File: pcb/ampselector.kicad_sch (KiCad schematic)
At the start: 24 parts, among them SW1 SW_Push, SW10 RotaryEncoder_Switch, SW2 SW_Push, SW3 SW_Push, SW4 SW_Push, SW5 SW_Push, SW6 SW_Push, SW7 SW_Push, SW8 SW_Push, SW9 RotaryEncoder_Switch, U1 MOUDLE-SEEEDUINO-XIAO, U2 ER_OLEDM0.91_1x-I2C

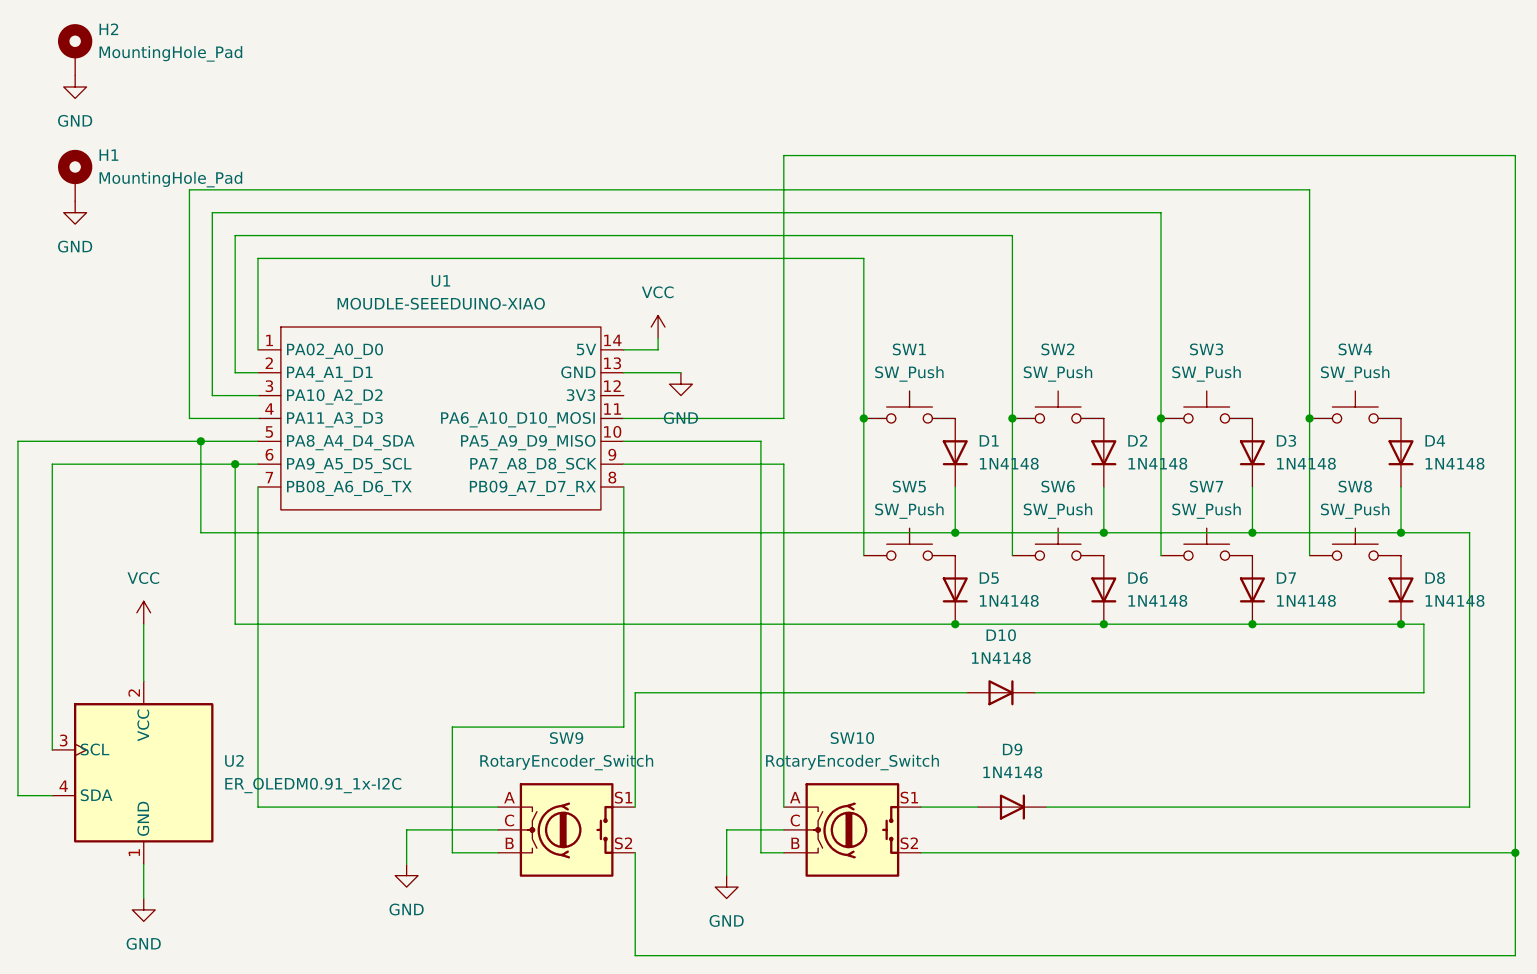
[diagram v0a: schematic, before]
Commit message: Designed Case
Signed-off-by: Ravinder Olivier Singh Dadiala <ravinder-Olivier@outlook.com>
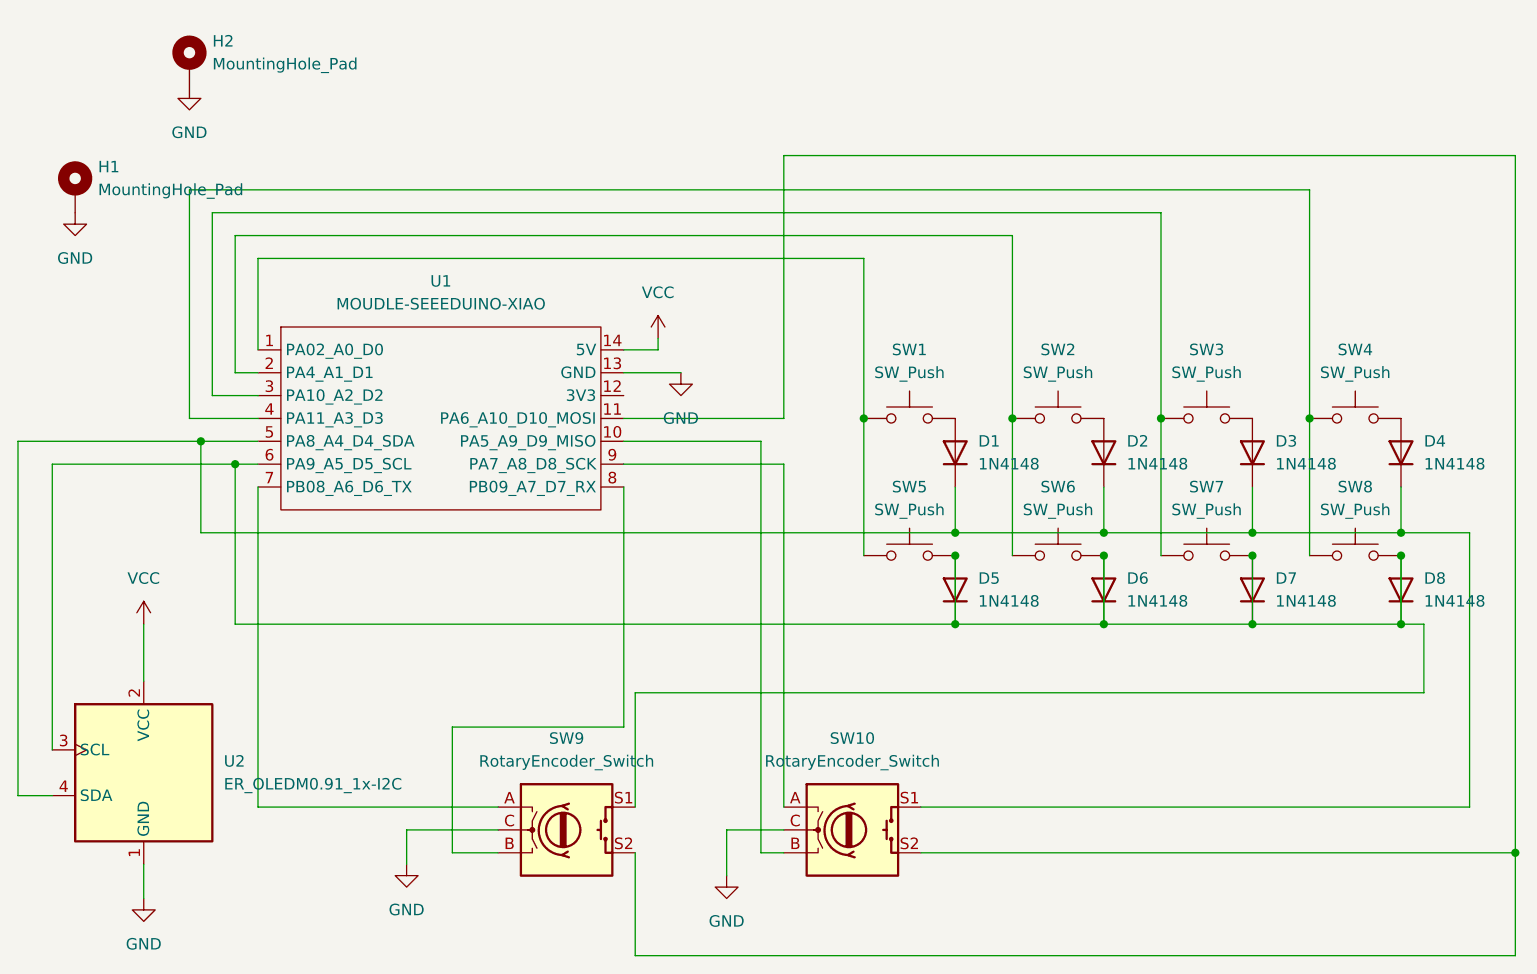
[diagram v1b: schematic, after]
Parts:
- removed D10, D9: 1N4148, Diode_THT:D_DO-35_SOD27_P7.62mm_Horizontal, symbol Diode:1N4148
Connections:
- net at D5.1 (K), D6.1 (K), D7.1 (K)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: now also D5.2 (A), D6.2 (A), D7.2 (A), D8.2 (A), SW5.2, SW6.2, SW7.2, SW8.2, SW9.S1
- net at D1.1 (K), D2.1 (K), D3.1 (K)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: now also SW10.S1
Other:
- moved on the sheet: H1, H2
